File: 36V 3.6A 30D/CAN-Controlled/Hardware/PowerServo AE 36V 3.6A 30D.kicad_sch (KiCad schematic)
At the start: 23 parts, among them J1 Control_In, J2 MOT_A, J3 Prog_IN, J4 Power_In, J6 Control_In, J7 MOT_B, U1 LMZM23601V5, U2 TLV76733DRVx, U3 DRV8871DDA, U4 MA730, U5 TJA1051T-3, U7 STM32G0B1KBTx

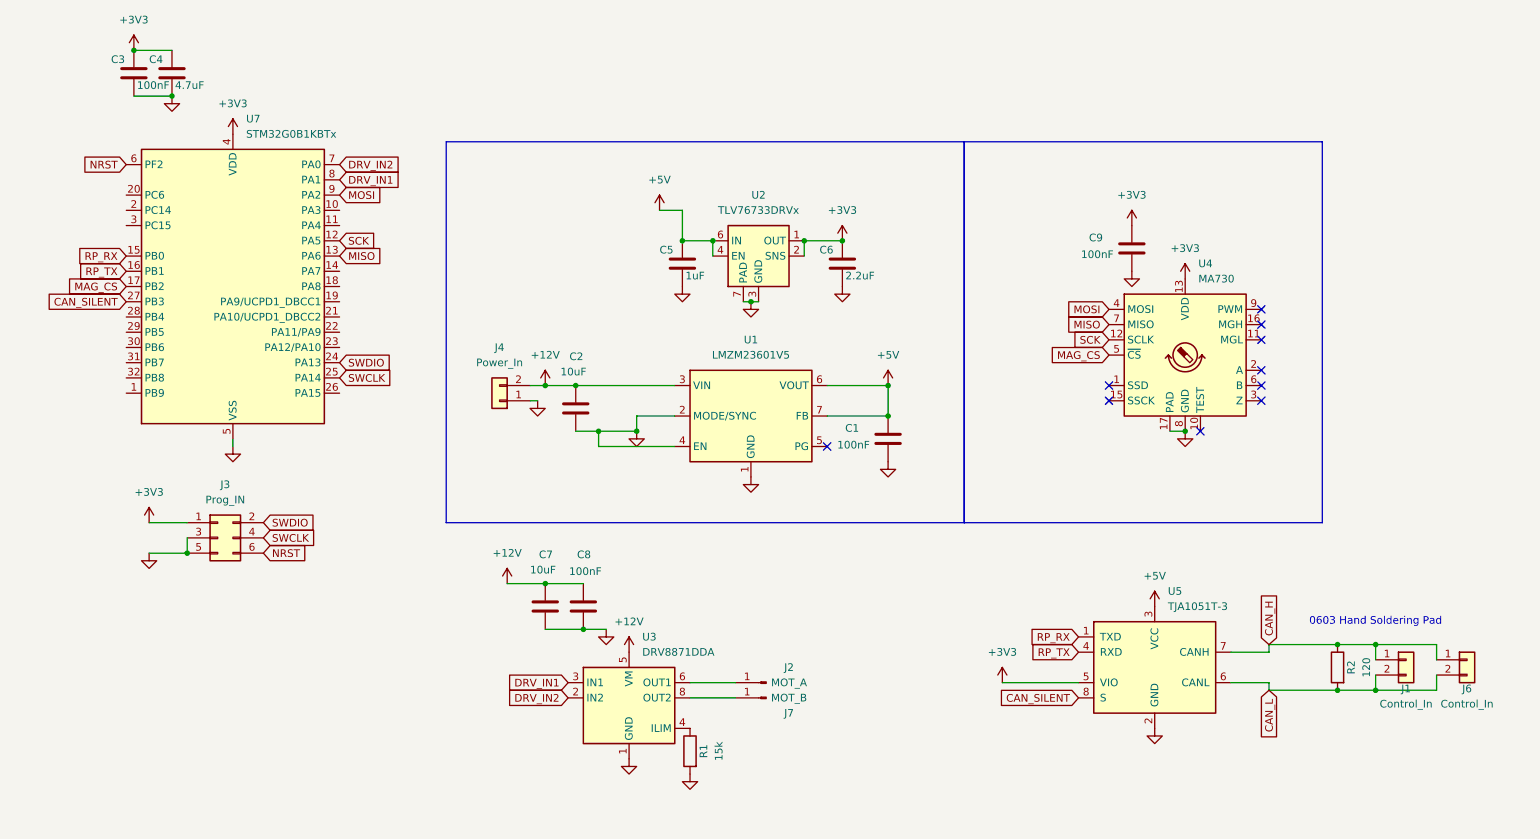
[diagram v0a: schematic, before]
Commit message: Review Request Files and Preparations
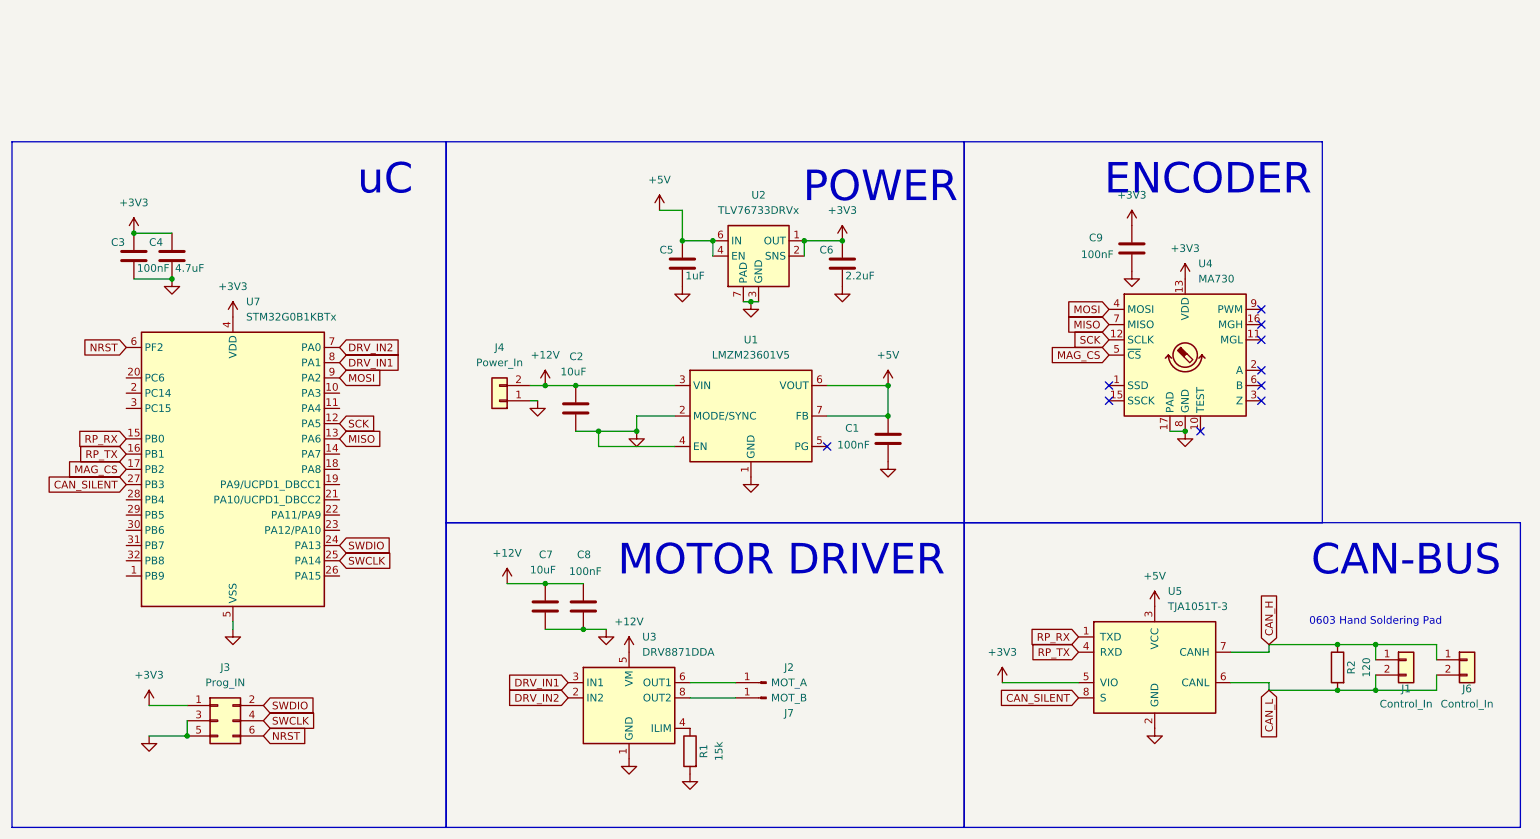
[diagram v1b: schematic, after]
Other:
- note added: "CAN-BUS"
- note added: "ENCODER"
- note added: "MOTOR DRIVER"
- note added: "POWER"
- note added: "uC"
- moved on the sheet: C3, C4, J3, U7
